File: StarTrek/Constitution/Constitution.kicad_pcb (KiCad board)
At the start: 2 copper layers, 1 part

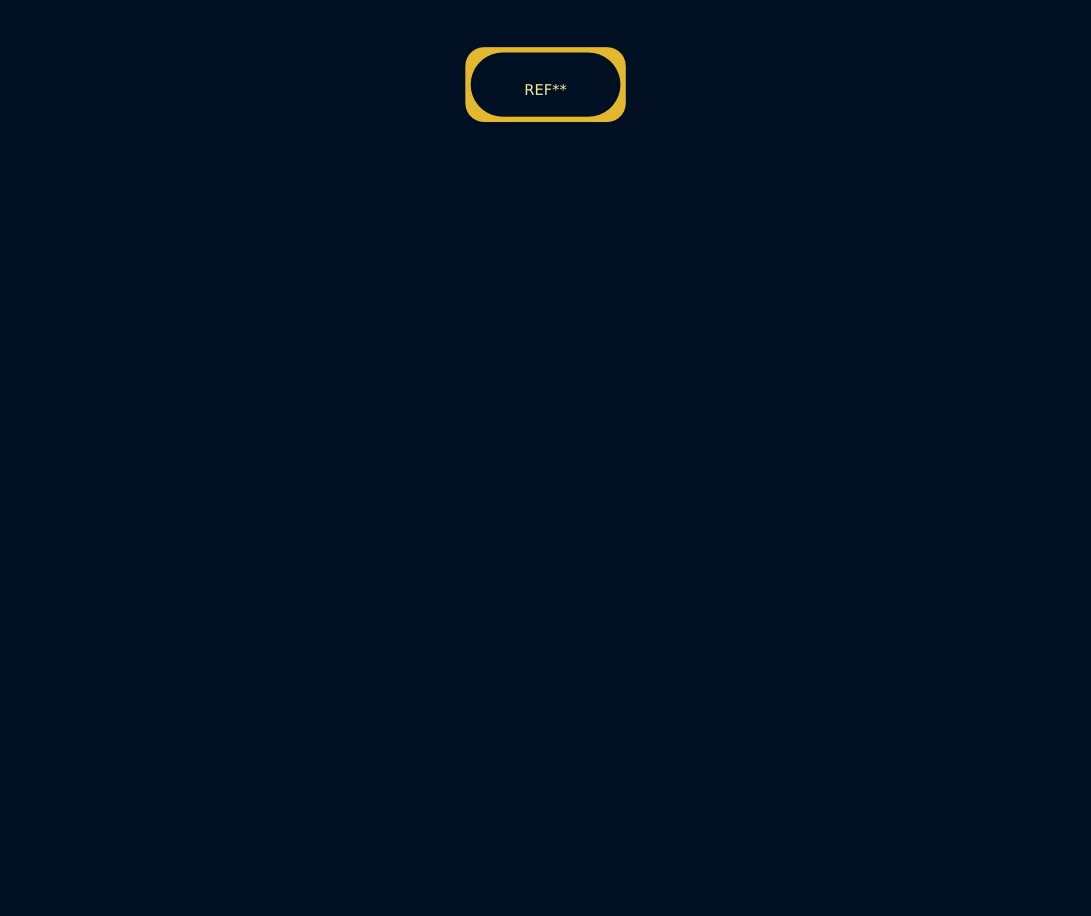
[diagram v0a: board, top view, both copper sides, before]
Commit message: Updates Constitution
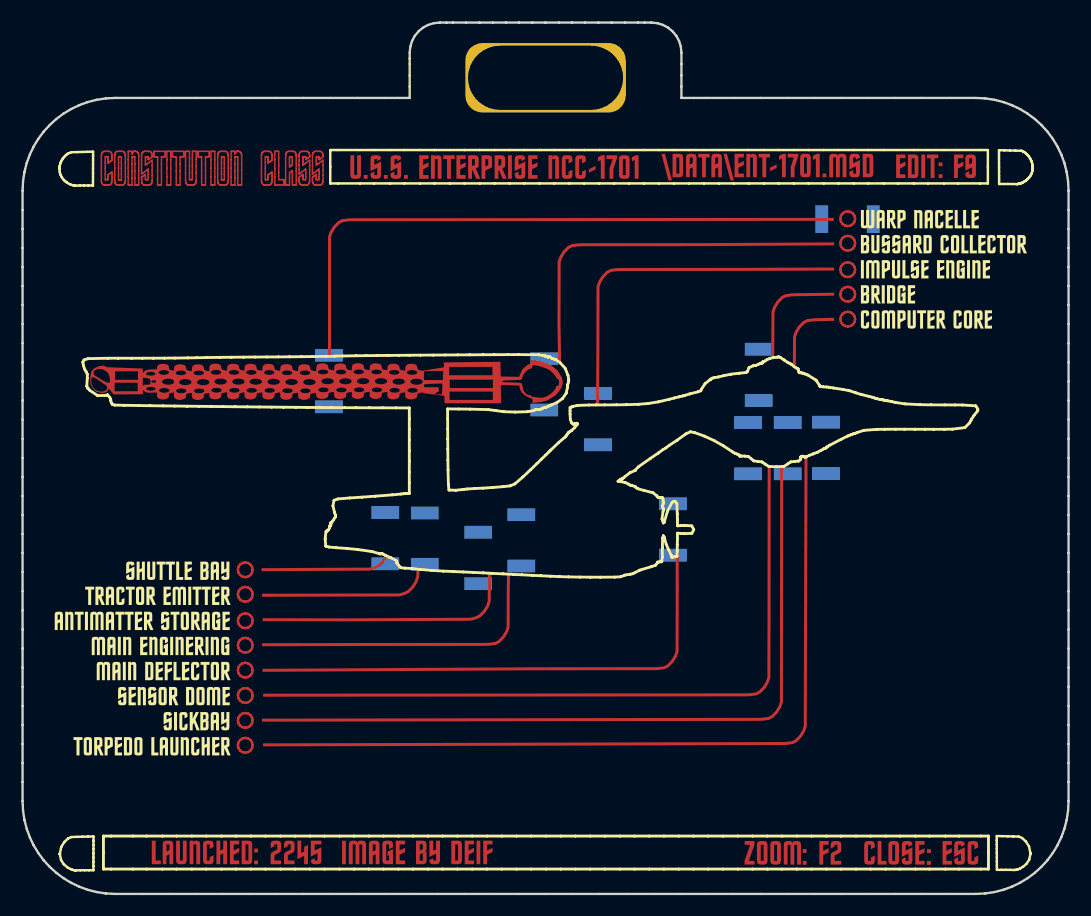
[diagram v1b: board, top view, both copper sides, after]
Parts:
- added LED**: Reverse_LWT773Q2R25K8LZ, constitution:Reverse_LWT773Q2R25K8LZ, B.Cu at (164.0, 103.2)
- added LED**: Reverse_LWT773Q2R25K8LZ, constitution:Reverse_LWT773Q2R25K8LZ, B.Cu at (131.5, 113.5)
- added LED**: Reverse_LWT773Q2R25K8LZ, constitution:Reverse_LWT773Q2R25K8LZ, B.Cu at (126.5, 111.7)
- added LED**: Reverse_LWT773Q2R25K8LZ, constitution:Reverse_LWT773Q2R25K8LZ, B.Cu at (122.8, 111.6)
- added LED**: Reverse_LWT773Q2R25K8LZ, constitution:Reverse_LWT773Q2R25K8LZ, B.Cu at (166.0, 81.8)
- added LED**: Reverse_LWT773Q2R25K8LZ, constitution:Reverse_LWT773Q2R25K8LZ, B.Cu at (156.7, 103.2)
- added LED**: Reverse_LWT773Q2R25K8LZ, constitution:Reverse_LWT773Q2R25K8LZ, B.Cu at (160.4, 103.2)
- added LED**: Reverse_LWT773Q2R25K8LZ, constitution:Reverse_LWT773Q2R25K8LZ, B.Cu at (157.7, 96.3)
- added LED**: Reverse_LWT773Q2R25K8LZ, constitution:Reverse_LWT773Q2R25K8LZ, B.Cu at (142.7, 100.5)
- added LED**: Reverse_LWT773Q2R25K8LZ, constitution:Reverse_LWT773Q2R25K8LZ, B.Cu at (149.7, 110.8)
- added LED**: Reverse_LWT773Q2R25K8LZ, constitution:Reverse_LWT773Q2R25K8LZ, B.Cu at (117.6, 96.9)
- added LED**: Reverse_LWT773Q2R25K8LZ, constitution:Reverse_LWT773Q2R25K8LZ, B.Cu at (137.7, 97.2)
- added LED**: Reverse_LWT773Q2R25K8LZ, constitution:Reverse_LWT773Q2R25K8LZ, B.Cu at (135.5, 111.8)
- added svg2mod: G***, constitution:Mask_Nave.01, F.Cu at (136.4, 104.9)
- added svg2mod: G***, constitution:Constitution.All.01, F.Cu at (137.8, 104.1)
- added svg2mod: G***, constitution:Engine.Cu.01, F.Cu at (114.9, 97.0)
- added svg2mod: G***, constitution:Engine2.Cu.01, F.Cu at (133.9, 97.0)
- added svg2mod: G***, constitution:Engine3.Cu.01, F.Cu at (100.8, 96.9)
- added svg2mod: G***, constitution:Engine4.Cu.01, F.Cu at (97.7, 96.8)
- moved REF** 0.64 mm to (137.8, 68.6)
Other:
- board outline added: 97.8 x 81.4 mm
